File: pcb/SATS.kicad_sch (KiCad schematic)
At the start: 27 parts, among them J1 Raspberry_Pi_2_3, J10 EXT_GPIO, J11 EXT_GPIO, J12 EXT_GPIO, J13 EXT_GPIO, J2 A00-432-262-450, J3 AudioJack4_SwitchTR1, J4 5V, J5 3.3V, J6 Card LED, J7 Wiegand, J8 Beep, J9 Card Power, SW1 Main Door Switch, SW2 Serv Door Switch, SW3 Third Reed Switch, U1 MCP23017_SP, U2 MCP23017_SP, U3 CD40109BE, U4 IRLZ14PBF

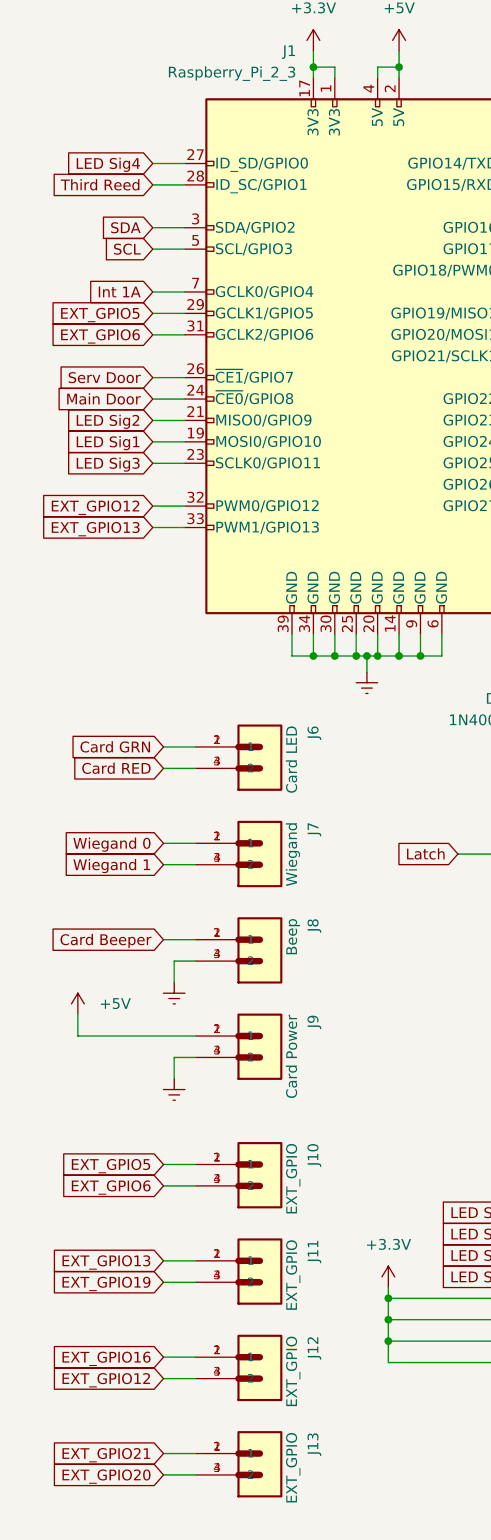
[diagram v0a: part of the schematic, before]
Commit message: mostly done
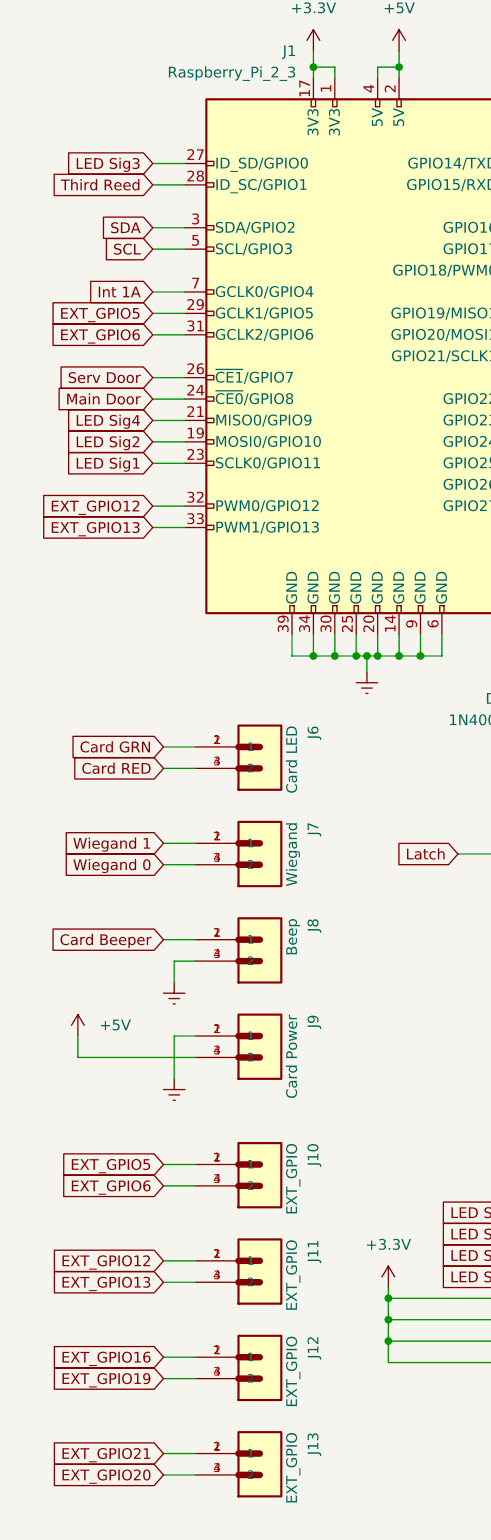
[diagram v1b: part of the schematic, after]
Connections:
- net +5V: now also J9.3 (2), J9.4 (2); no longer J9.1, J9.2 (1)
- net EXT_GPIO12: now also J11.1, J11.2 (1); no longer J12.3 (2), J12.4 (2)
- net EXT_GPIO13: now also J11.3 (2), J11.4 (2); no longer J11.1, J11.2 (1)
- net EXT_GPIO19: now also J12.3 (2), J12.4 (2); no longer J11.3 (2), J11.4 (2)
- net Earth: now also J9.1, J9.2 (1); no longer J9.3 (2), J9.4 (2)
- net LED Sig1: now also J1.23 (SCLK0/GPIO11); no longer J1.19 (MOSI0/GPIO10)
- net LED Sig2: now also J1.19 (MOSI0/GPIO10); no longer J1.21 (MISO0/GPIO9)
- net LED Sig3: now also J1.27 (ID_SD/GPIO0); no longer J1.23 (SCLK0/GPIO11)
- net LED Sig4: now also J1.21 (MISO0/GPIO9); no longer J1.27 (ID_SD/GPIO0)
- net Wiegand 0: now also J7.3 (2), J7.4 (2); no longer J7.1, J7.2 (1)
- net Wiegand 1: now also J7.1, J7.2 (1); no longer J7.3 (2), J7.4 (2)
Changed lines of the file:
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@@
     (stroke (width 0) (type default) (color 0 0 0 0))
   )
-  (wire (pts (xy 20.32 138.43) (xy 34.29 138.43))
+  (wire (pts (xy 20.32 140.97) (xy 34.29 140.97))
     (stroke (width 0) (type default) (color 0 0 0 0))
   )
@@
     (stroke (width 0) (type default) (color 0 0 0 0))
   )
-  (wire (pts (xy 31.75 140.97) (xy 31.75 143.51))
+  (wire (pts (xy 31.75 138.43) (xy 31.75 143.51))
     (stroke (width 0) (type default) (color 0 0 0 0))
   )
@@
     (stroke (width 0) (type default) (color 0 0 0 0))
   )
-  (wire (pts (xy 31.75 140.97) (xy 34.29 140.97))
+  (wire (pts (xy 31.75 138.43) (xy 34.29 138.43))
     (stroke (width 0) (type default) (color 0 0 0 0))
   )
@@
     (stroke (width 0) (type default) (color 0 0 0 0))
   )
-  (wire (pts (xy 20.32 135.89) (xy 20.32 138.43))
+  (wire (pts (xy 20.32 138.43) (xy 20.32 140.97))
     (stroke (width 0) (type default) (color 0 0 0 0))
   )
@@
     )
   )
-  (global_label "LED Sig3" (shape input) (at 29.21 70.485 180) (fields_autoplaced)
+  (global_label "LED Sig3" (shape input) (at 29.21 34.925 180) (fields_autoplaced)
+    (effects (font (size 1.27 1.27)) (justify right))
+    (property "Intersheet References" "${INTERSHEET_REFS}" (id 0) (at 18.2093 35.0044 0)
+      (effects (font (size 1.27 1.27)) (justify right) hide)
+    )
+  )
+  (global_label "LED Sig1" (shape input) (at 29.21 70.485 180) (fields_autoplaced)
     (effects (font (size 1.27 1.27)) (justify right))
     (property "Intersheet References" "${INTERSHEET_REFS}" (id 0) (at 18.2093 70.4056 0)
@@
     )
   )
-  (global_label "LED Sig1" (shape input) (at 29.21 67.945 180) (fields_autoplaced)
-    (effects (font (size 1.27 1.27)) (justify right))
-    (property "Intersheet References" "${INTERSHEET_REFS}" (id 0) (at 18.2093 67.8656 0)
-      (effects (font (size 1.27 1.27)) (justify right) hide)
-    )
-  )
-  (global_label "Wiegand 0" (shape input) (at 30.48 115.57 180) (fields_autoplaced)
-    (effects (font (size 1.27 1.27)) (justify right))
-    (property "Intersheet References" "${INTERSHEET_REFS}" (id 0) (at 18.1488 115.4906 0)
+  (global_label "Wiegand 0" (shape input) (at 30.48 118.11 180) (fields_autoplaced)
+    (effects (font (size 1.27 1.27)) (justify right))
+    (property "Intersheet References" "${INTERSHEET_REFS}" (id 0) (at 18.1488 118.1894 0)
       (effects (font (size 1.27 1.27)) (justify right) hide)
     )
@@
     )
   )
-  (global_label "EXT_GPIO12" (shape input) (at 30.48 179.07 180) (fields_autoplaced)
-    (effects (font (size 1.27 1.27)) (justify right))
-    (property "Intersheet References" "${INTERSHEET_REFS}" (id 0) (at 16.8788 178.9906 0)
+  (global_label "EXT_GPIO12" (shape input) (at 30.48 165.1 180) (fields_autoplaced)
+    (effects (font (size 1.27 1.27)) (justify right))
+    (property "Intersheet References" "${INTERSHEET_REFS}" (id 0) (at 16.8788 165.0206 0)
       (effects (font (size 1.27 1.27)) (justify right) hide)
     )
@@
     )
   )
-  (global_label "EXT_GPIO13" (shape input) (at 30.48 165.1 180) (fields_autoplaced)
-    (effects (font (size 1.27 1.27)) (justify right))
-    (property "Intersheet References" "${INTERSHEET_REFS}" (id 0) (at 16.8788 165.0206 0)
+  (global_label "EXT_GPIO13" (shape input) (at 30.48 167.64 180) (fields_autoplaced)
+    (effects (font (size 1.27 1.27)) (justify right))
+    (property "Intersheet References" "${INTERSHEET_REFS}" (id 0) (at 16.8788 167.7194 0)
       (effects (font (size 1.27 1.27)) (justify right) hide)
     )
@@
     )
   )
-  (global_label "EXT_GPIO19" (shape input) (at 30.48 167.64 180) (fields_autoplaced)
-    (effects (font (size 1.27 1.27)) (justify right))
-    (property "Intersheet References" "${INTERSHEET_REFS}" (id 0) (at 16.8788 167.5606 0)
+  (global_label "EXT_GPIO19" (shape input) (at 30.48 179.07 180) (fields_autoplaced)
+    (effects (font (size 1.27 1.27)) (justify right))
+    (property "Intersheet References" "${INTERSHEET_REFS}" (id 0) (at 16.8788 179.1494 0)
       (effects (font (size 1.27 1.27)) (justify right) hide)
     )
@@
     )
   )
-  (global_label "Wiegand 1" (shape input) (at 30.48 118.11 180) (fields_autoplaced)
-    (effects (font (size 1.27 1.27)) (justify right))
-    (property "Intersheet References" "${INTERSHEET_REFS}" (id 0) (at 18.1488 118.0306 0)
+  (global_label "Wiegand 1" (shape input) (at 30.48 115.57 180) (fields_autoplaced)
+    (effects (font (size 1.27 1.27)) (justify right))
+    (property "Intersheet References" "${INTERSHEET_REFS}" (id 0) (at 18.1488 115.6494 0)
       (effects (font (size 1.27 1.27)) (justify right) hide)
     )
@@
     )
   )
-  (global_label "LED Sig4" (shape input) (at 29.21 34.925 180) (fields_autoplaced)
-    (effects (font (size 1.27 1.27)) (justify right))
-    (property "Intersheet References" "${INTERSHEET_REFS}" (id 0) (at 18.2093 34.8456 0)
+  (global_label "LED Sig4" (shape input) (at 29.21 65.405 180) (fields_autoplaced)
+    (effects (font (size 1.27 1.27)) (justify right))
+    (property "Intersheet References" "${INTERSHEET_REFS}" (id 0) (at 18.2093 65.3256 0)
       (effects (font (size 1.27 1.27)) (justify right) hide)
     )
@@
     )
   )
-  (global_label "LED Sig2" (shape input) (at 29.21 65.405 180) (fields_autoplaced)
-    (effects (font (size 1.27 1.27)) (justify right))
-    (property "Intersheet References" "${INTERSHEET_REFS}" (id 0) (at 18.2093 65.3256 0)
+  (global_label "LED Sig2" (shape input) (at 29.21 67.945 180) (fields_autoplaced)
+    (effects (font (size 1.27 1.27)) (justify right))
+    (property "Intersheet References" "${INTERSHEET_REFS}" (id 0) (at 18.2093 68.0244 0)
       (effects (font (size 1.27 1.27)) (justify right) hide)
     )
@@
     (pin "1")
   )
-  (symbol (lib_id "power:+5V") (at 20.32 135.89 0) (mirror y) (unit 1)
-    (in_bom yes) (on_board yes) (fields_autoplaced)
-    (property "Reference" "#PWR0135" (id 0) (at 20.32 139.7 0)
-      (effects (font (size 1.27 1.27)) hide)
-    )
-    (property "Value" "+5V" (id 1) (at 22.86 134.6199 0)
-      (effects (font (size 1.27 1.27)) (justify right))
-    )
-    (property "Footprint" "" (id 2) (at 20.32 135.89 0)
-      (effects (font (size 1.27 1.27)) hide)
-    )
-    (property "Datasheet" "" (id 3) (at 20.32 135.89 0)
-      (effects (font (size 1.27 1.27)) hide)
-    )
+  (symbol (lib_id "power:+5V") (at 20.32 138.43 0) (mirror y) (unit 1)
+    (in_bom yes) (on_board yes) (fields_autoplaced)
+    (property "Reference" "#PWR0135" (id 0) (at 20.32 142.24 0)
+      (effects (font (size 1.27 1.27)) hide)
+    )
+    (property "Value" "+5V" (id 1) (at 22.86 137.1599 0)
+      (effects (font (size 1.27 1.27)) (justify right))
+    )
+    (property "Footprint" "" (id 2) (at 20.32 138.43 0)
+      (effects (font (size 1.27 1.27)) hide)
+    )
+    (property "Datasheet" "" (id 3) (at 20.32 138.43 0)
+      (effects (font (size 1.27 1.27)) hide)
+    )
